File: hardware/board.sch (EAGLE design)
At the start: 17 parts, among them IC1 MCP4131, IC2 L272, Q1 BC638, Q3 BC638

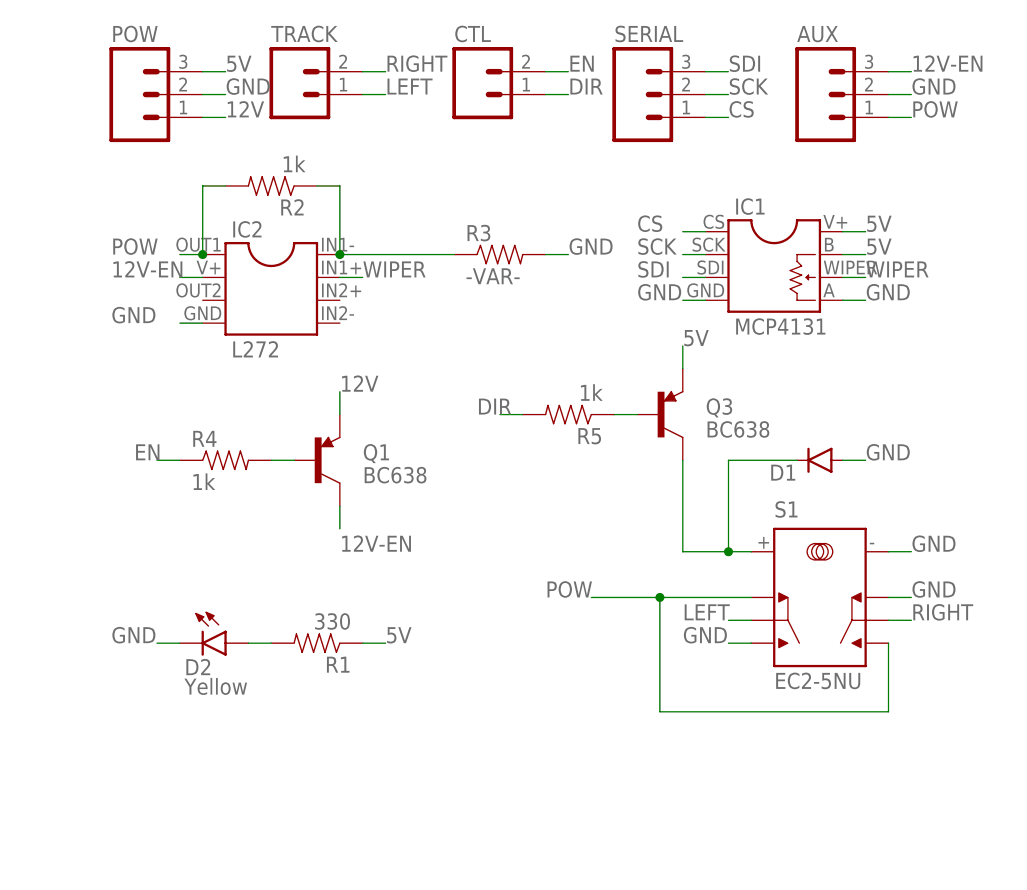
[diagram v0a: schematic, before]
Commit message: renaming things, adding images
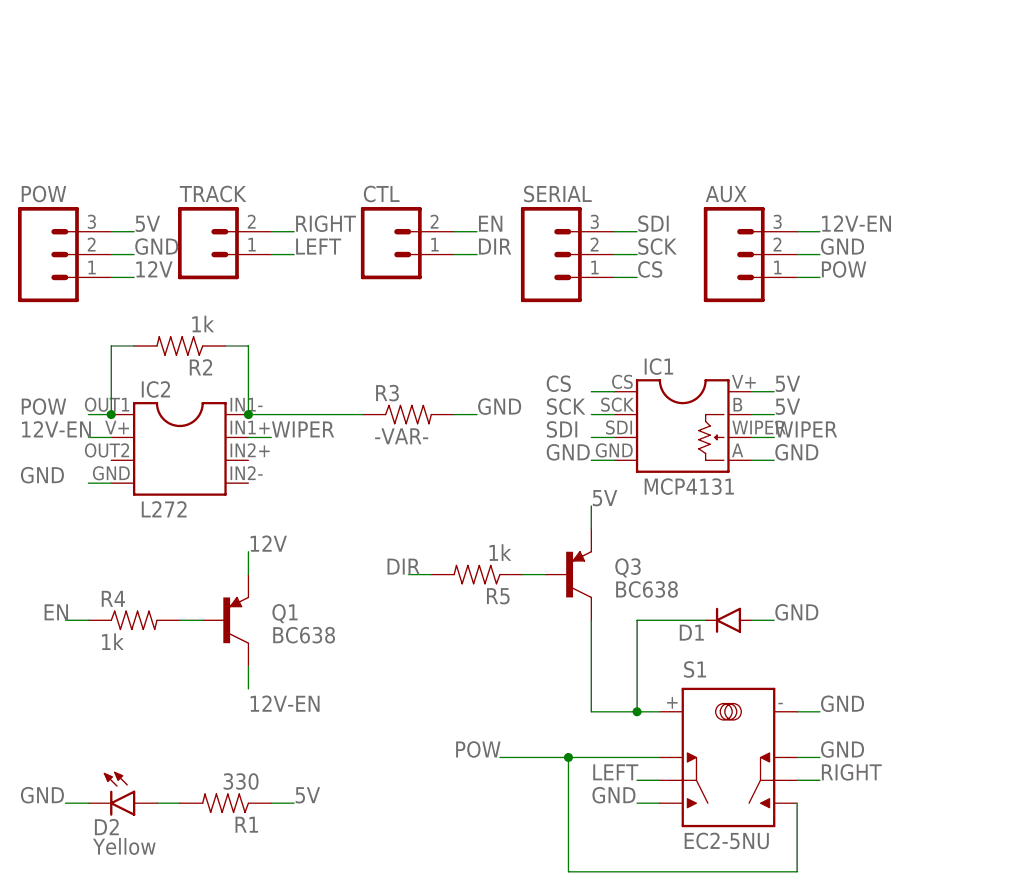
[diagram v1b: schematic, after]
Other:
- moved on the sheet: AUX, CTL, D1, D2, IC1, IC2, POW, Q1, Q3, R1, R2, R3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
